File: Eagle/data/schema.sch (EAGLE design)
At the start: 9 parts, among them IC1 PICAXE-08M2-DIL, K1 ARK500/2

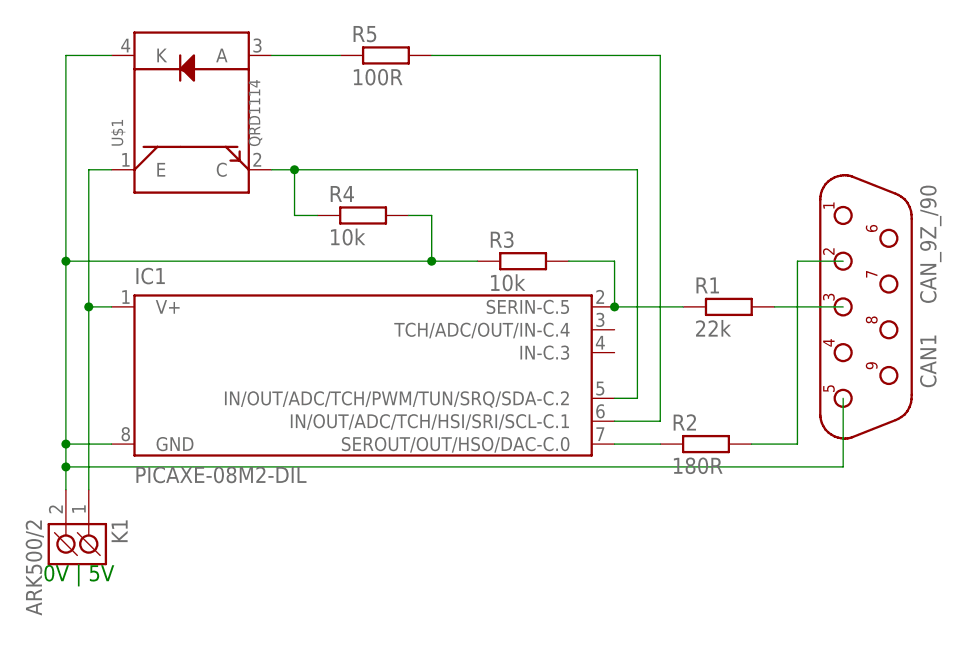
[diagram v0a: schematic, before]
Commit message: Úprava souborů pro SW Eagle
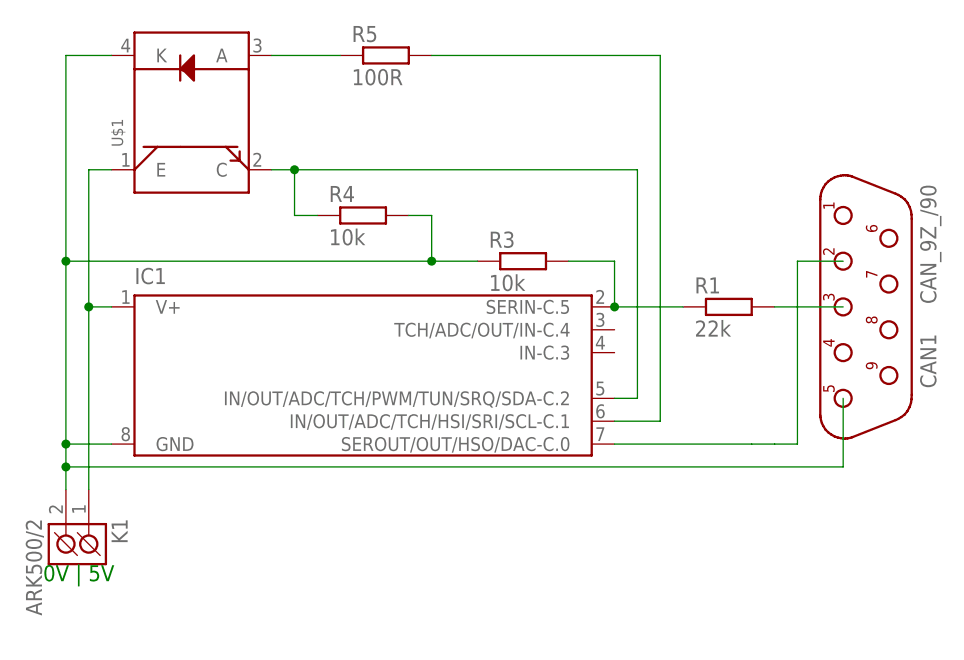
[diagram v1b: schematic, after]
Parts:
- removed R2: 180R, eagle-ltspice:R0207/10
- IC1: device PICAXE:PICAXE-08M2-DIL -> RONJA:PICAXE-08M2-DIL
- U$1: device SparkFun:QRD1114 -> RONJA:QRD1114
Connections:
- removed net N$3: CAN1.2, R2.2
- net N$1: now also CAN1.2; no longer R2.1
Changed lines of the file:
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@@
 </classes>
 <parts>
-<part name="IC1" library="PICAXE" deviceset="PICAXE-08M2" device="-DIL"/>
 <part name="R1" library="eagle-ltspice" deviceset="R" device="0207/10" value="22k"/>
-<part name="R2" library="eagle-ltspice" deviceset="R" device="0207/10" value="180R"/>
 <part name="R3" library="eagle-ltspice" deviceset="R" device="0207/10" value="10k"/>
-<part name="U$1" library="SparkFun" deviceset="QRD1114" device=""/>
 <part name="R4" library="eagle-ltspice" deviceset="R" device="0207/10" value="10k"/>
 <part name="R5" library="eagle-ltspice" deviceset="R" device="0207/10" value="100R"/>
 <part name="K1" library="#PaJa_konektory" deviceset="ARK500/2" device=""/>
 <part name="CAN1" library="#PaJa_konektory" deviceset="CAN_9Z" device="_/90"/>
+<part name="U$1" library="RONJA" deviceset="QRD1114" device=""/>
+<part name="IC1" library="RONJA" deviceset="PICAXE-08M2" device="-DIL"/>
 </parts>
 <sheets>
@@
 </plain>
 <instances>
-<instance part="IC1" gate="G$1" x="60.96" y="86.36"/>
 <instance part="R1" gate="G$1" x="101.6" y="93.98"/>
-<instance part="R2" gate="G$1" x="99.06" y="78.74"/>
 <instance part="R3" gate="G$1" x="78.74" y="99.06"/>
-<instance part="U$1" gate="G$1" x="43.18" y="111.76" rot="MR90"/>
 <instance part="R4" gate="G$1" x="60.96" y="104.14"/>
 <instance part="R5" gate="G$1" x="63.5" y="121.92"/>
 <instance part="K1" gate="K" x="30.48" y="68.58" rot="R270"/>
 <instance part="CAN1" gate="CAN" x="116.84" y="93.98" rot="R90"/>
+<instance part="U$1" gate="G$1" x="43.18" y="111.76" rot="MR90"/>
+<instance part="IC1" gate="G$1" x="60.96" y="86.36"/>
 </instances>
 <busses>
@@
 <segment>
 <pinref part="IC1" gate="G$1" pin="SEROUT/OUT/HSO/DAC-C.0@7"/>
-<pinref part="R2" gate="G$1" pin="1"/>
-<wire x1="88.9" y1="78.74" x2="93.98" y2="78.74" width="0.1524" layer="91"/>
+<wire x1="104.14" y1="78.74" x2="106.68" y2="78.74" width="0.1524" layer="91"/>
+<wire x1="106.68" y1="78.74" x2="109.22" y2="78.74" width="0.1524" layer="91"/>
+<wire x1="109.22" y1="78.74" x2="109.22" y2="99.06" width="0.1524" layer="91"/>
+<pinref part="CAN1" gate="CAN" pin="2"/>
+<wire x1="109.22" y1="99.06" x2="114.3" y2="99.06" width="0.1524" layer="91"/>
+<wire x1="88.9" y1="78.74" x2="104.14" y2="78.74" width="0.1524" layer="91"/>
 </segment>
 </net>
@@
 </segment>
 </net>
-<net name="N$3" class="0">
-<segment>
-<pinref part="R2" gate="G$1" pin="2"/>
-<wire x1="104.14" y1="78.74" x2="109.22" y2="78.74" width="0.1524" layer="91"/>
-<wire x1="109.22" y1="78.74" x2="109.22" y2="99.06" width="0.1524" layer="91"/>
-<pinref part="CAN1" gate="CAN" pin="2"/>
-<wire x1="109.22" y1="99.06" x2="114.3" y2="99.06" width="0.1524" layer="91"/>
-</segment>
-</net>
 <net name="N$10" class="0">
 <segment>
 <pinref part="R1" gate="G$1" pin="1"/>
-<pinref part="IC1" gate="G$1" pin="SERIN-C.5@2"/>
 <wire x1="88.9" y1="93.98" x2="96.52" y2="93.98" width="0.1524" layer="91"/>
 <wire x1="88.9" y1="99.06" x2="88.9" y2="93.98" width="0.1524" layer="91"/>
-<junction x="88.9" y="93.98"/>
 <pinref part="R3" gate="G$1" pin="2"/>
 <wire x1="83.82" y1="99.06" x2="88.9" y2="99.06" width="0.1524" layer="91"/>
+<pinref part="IC1" gate="G$1" pin="SERIN-C.5@2"/>
+<junction x="88.9" y="93.98"/>
 </segment>
 </net>
 <net name="N$9" class="0">
 <segment>
-<pinref part="IC1" gate="G$1" pin="V+@1"/>
 <wire x1="33.02" y1="93.98" x2="30.48" y2="93.98" width="0.1524" layer="91"/>
 <pinref part="K1" gate="K" pin="K1"/>
 <wire x1="30.48" y1="93.98" x2="30.48" y2="73.66" width="0.1524" layer="91"/>
-<wire x1="30.48" y1="93.98" x2="30.48" y2="109.22" width="0.1524" layer="91"/>
 <junction x="30.48" y="93.98"/>
 <pinref part="U$1" gate="G$1" pin="E"/>
+<wire x1="30.48" y1="93.98" x2="30.48" y2="109.22" width="0.1524" layer="91"/>
 <wire x1="30.48" y1="109.22" x2="33.02" y2="109.22" width="0.1524" layer="91"/>
+<pinref part="IC1" gate="G$1" pin="V+@1"/>
 </segment>
 </net>
 <net name="N$4" class="0">
 <segment>
-<pinref part="U$1" gate="G$1" pin="A"/>
 <pinref part="R5" gate="G$1" pin="1"/>
 <wire x1="50.8" y1="121.92" x2="58.42" y2="121.92" width="0.1524" layer="91"/>
+<pinref part="U$1" gate="G$1" pin="A"/>
 </segment>
 </net>
 <net name="N$5" class="0">
 <segment>
-<pinref part="IC1" gate="G$1" pin="IN/OUT/ADC/TCH/HSI/SRI/SCL-C.1@6"/>
 <wire x1="88.9" y1="81.28" x2="93.98" y2="81.28" width="0.1524" layer="91"/>
 <wire x1="93.98" y1="81.28" x2="93.98" y2="121.92" width="0.1524" layer="91"/>
 <pinref part="R5" gate="G$1" pin="2"/>
 <wire x1="93.98" y1="121.92" x2="68.58" y2="121.92" width="0.1524" layer="91"/>
+<pinref part="IC1" gate="G$1" pin="IN/OUT/ADC/TCH/HSI/SRI/SCL-C.1@6"/>
 </segment>
 </net>
 <net name="N$6" class="0">
 <segment>
-<pinref part="U$1" gate="G$1" pin="C"/>
 <wire x1="50.8" y1="109.22" x2="53.34" y2="109.22" width="0.1524" layer="91"/>
 <wire x1="53.34" y1="109.22" x2="91.44" y2="109.22" width="0.1524" layer="91"/>
 <wire x1="91.44" y1="109.22" x2="91.44" y2="83.82" width="0.1524" layer="91"/>
-<pinref part="IC1" gate="G$1" pin="IN/OUT/ADC/TCH/PWM/TUN/SRQ/SDA-C.2@5"/>
 <wire x1="91.44" y1="83.82" x2="88.9" y2="83.82" width="0.1524" layer="91"/>
-<wire x1="53.34" y1="109.22" x2="53.34" y2="104.14" width="0.1524" layer="91"/>
-<junction x="53.34" y="109.22"/>
 <pinref part="R4" gate="G$1" pin="1"/>
 <wire x1="55.88" y1="104.14" x2="53.34" y2="104.14" width="0.1524" layer="91"/>
+<pinref part="U$1" gate="G$1" pin="C"/>
+<wire x1="53.34" y1="104.14" x2="53.34" y2="109.22" width="0.1524" layer="91"/>
+<junction x="53.34" y="109.22"/>
+<pinref part="IC1" gate="G$1" pin="IN/OUT/ADC/TCH/PWM/TUN/SRQ/SDA-C.2@5"/>
 </segment>
 </net>
@@
 <wire x1="68.58" y1="99.06" x2="27.94" y2="99.06" width="0.1524" layer="91"/>
 <wire x1="27.94" y1="99.06" x2="27.94" y2="78.74" width="0.1524" layer="91"/>
-<pinref part="IC1" gate="G$1" pin="GND@8"/>
 <wire x1="33.02" y1="78.74" x2="27.94" y2="78.74" width="0.1524" layer="91"/>
 <junction x="27.94" y="78.74"/>
@@
 <wire x1="27.94" y1="76.2" x2="27.94" y2="73.66" width="0.1524" layer="91"/>
 <junction x="27.94" y="76.2"/>
+<junction x="27.94" y="99.06"/>
 <wire x1="27.94" y1="99.06" x2="27.94" y2="121.92" width="0.1524" layer="91"/>
-<junction x="27.94" y="99.06"/>
-<pinref part="U$1" gate="G$1" pin="K"/>
 <wire x1="27.94" y1="121.92" x2="33.02" y2="121.92" width="0.1524" layer="91"/>
 <wire x1="68.58" y1="104.14" x2="68.58" y2="99.06" width="0.1524" layer="91"/>
@@
 <wire x1="68.58" y1="99.06" x2="73.66" y2="99.06" width="0.1524" layer="91"/>
 <junction x="68.58" y="99.06"/>
+<pinref part="U$1" gate="G$1" pin="K"/>
+<pinref part="IC1" gate="G$1" pin="GND@8"/>
 </segment>
 </net>
